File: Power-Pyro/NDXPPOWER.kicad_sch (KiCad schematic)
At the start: 0 parts

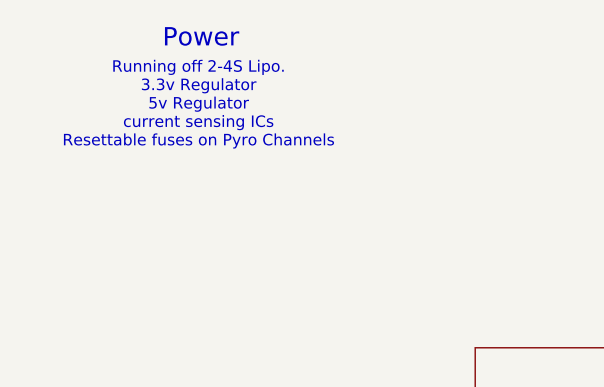
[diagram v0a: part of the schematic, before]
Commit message: 🔌
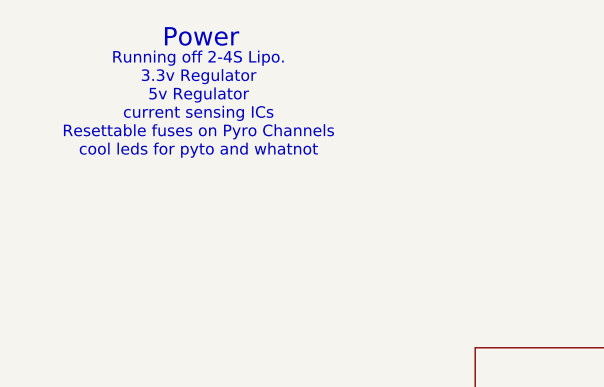
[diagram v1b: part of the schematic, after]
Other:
- note added: "Running off 2-4S Lipo. 3.3v Regulator 5v Regulator current sensing ICs Resettable fuses on Pyro Channels cool leds for pyto and whatnot"
- note removed: "Running off 2-4S Lipo. 3.3v Regulator 5v Regulator current sensing ICs Resettable fuses on Pyro Channels"
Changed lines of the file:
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@@
 		)
 	)
-	(text "Running off 2-4S Lipo.\n3.3v Regulator\n5v Regulator\ncurrent sensing ICs\nResettable fuses on Pyro Channels"
+	(text "Running off 2-4S Lipo.\n3.3v Regulator\n5v Regulator\ncurrent sensing ICs\nResettable fuses on Pyro Channels\ncool leds for pyto and whatnot\n"
 		(exclude_from_sim no)
 		(at 35.306 31.496 0)
